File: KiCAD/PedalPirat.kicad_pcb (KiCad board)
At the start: 2 copper layers, 55 parts, among them IC1 IS31CS8979-QFLS2-TR, IC2 IS32IO1028A-GRLA2-TR

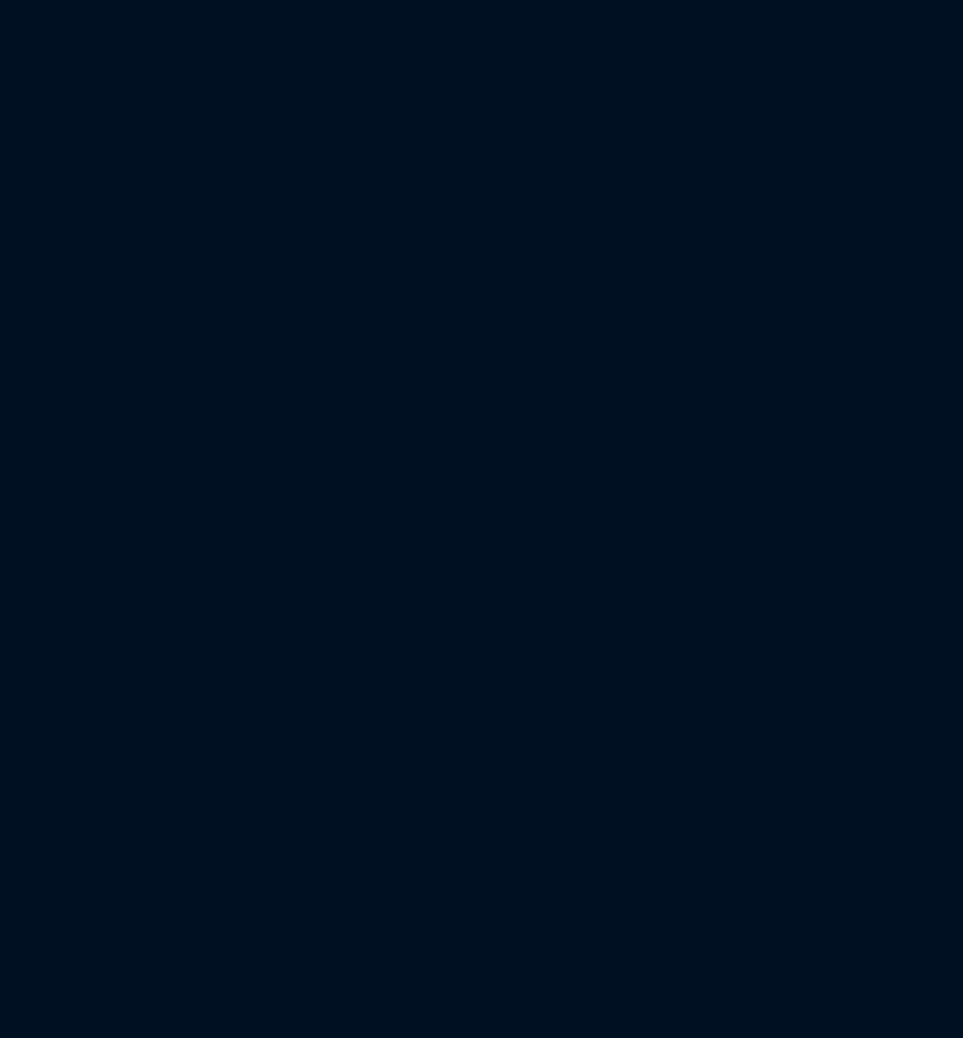
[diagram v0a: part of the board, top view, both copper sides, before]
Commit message: dasasd
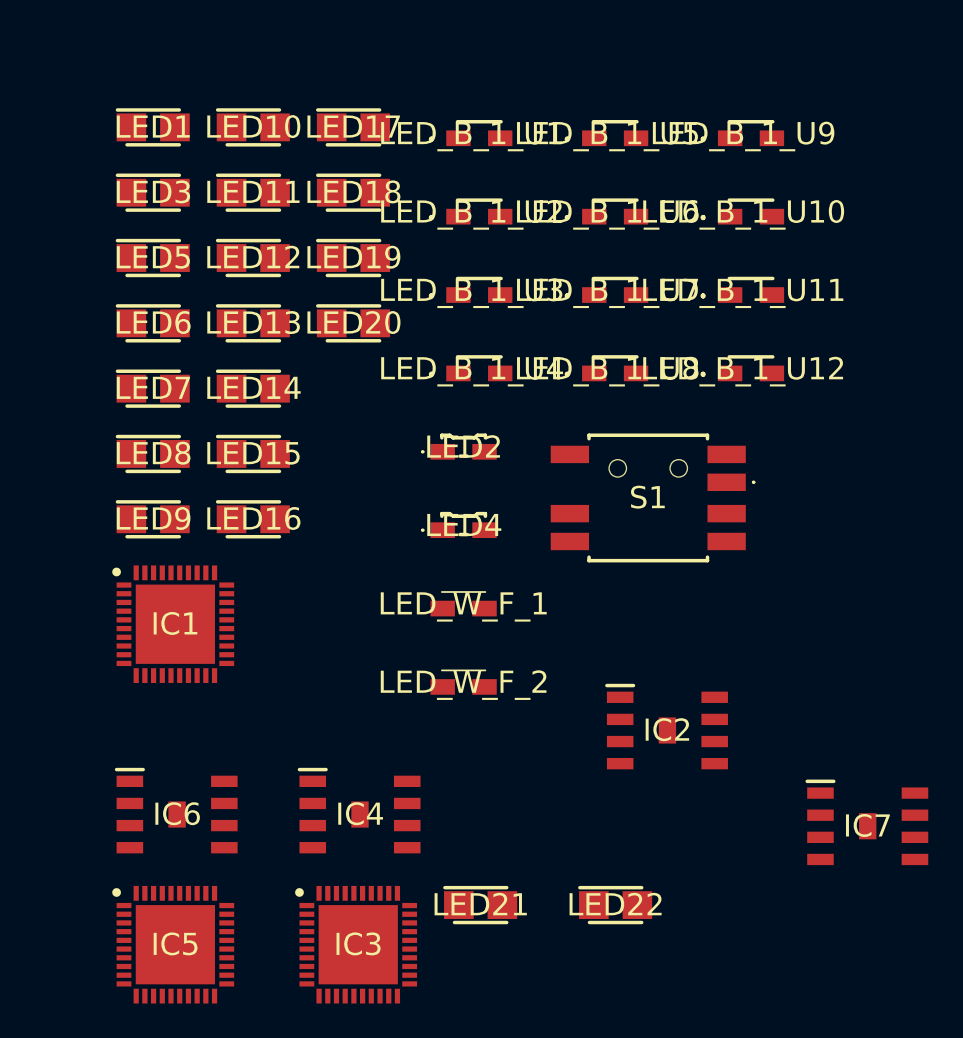
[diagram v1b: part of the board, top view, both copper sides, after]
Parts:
- added IC1: IS31CS8979-QFLS2-TR, SamacSys_Parts:QFN50P600X600X80-41N-D, F.Cu at (221.8, 97.4)
- added IC2: IS32IO1028A-GRLA2-TR, SamacSys_Parts:SOIC127P600X170-9N, F.Cu at (250.0, 103.5)
- added IC3: IS31CS8979-QFLS2-TR, SamacSys_Parts:QFN50P600X600X80-41N-D, F.Cu at (232.2, 115.8)
- added IC4: IS32IO1028A-GRLA2-TR, SamacSys_Parts:SOIC127P600X170-9N, F.Cu at (232.3, 108.3)
- added IC5: IS31CS8979-QFLS2-TR, SamacSys_Parts:QFN50P600X600X80-41N-D, F.Cu at (221.8, 115.8)
- added IC6: IS32IO1028A-GRLA2-TR, SamacSys_Parts:SOIC127P600X170-9N, F.Cu at (221.8, 108.3)
- added IC7: IS32LT3183A-GRLA3-TR, SamacSys_Parts:SOIC127P600X170-9N, F.Cu at (261.5, 109.0)
- added LED1: AA3021SESK_J3-TR, SamacSys_Parts:LEDM3020X150N, F.Cu at (220.5, 68.9)
- added LED10: AA3021SYSK_J3-TR, SamacSys_Parts:LEDM3020X150N, F.Cu at (226.2, 68.9)
- added LED11: AA3021SYSK_J3-TR, SamacSys_Parts:LEDM3020X150N, F.Cu at (226.2, 72.6)
- added LED12: AA3021SYSK_J3-TR, SamacSys_Parts:LEDM3020X150N, F.Cu at (226.2, 76.4)
- added LED13: AA3021SESK_J3-TR, SamacSys_Parts:LEDM3020X150N, F.Cu at (226.2, 80.1)
- added LED14: AA3021SYSK_J3-TR, SamacSys_Parts:LEDM3020X150N, F.Cu at (226.2, 83.9)
- added LED15: AA3021SYSK_J3-TR, SamacSys_Parts:LEDM3020X150N, F.Cu at (226.2, 87.6)
- added LED16: AA3021SYSK_J3-TR, SamacSys_Parts:LEDM3020X150N, F.Cu at (226.2, 91.4)
- added LED17: AA3021SYSK_J3-TR, SamacSys_Parts:LEDM3020X150N, F.Cu at (232.0, 68.9)
- added LED18: AA3021SYSK_J3-TR, SamacSys_Parts:LEDM3020X150N, F.Cu at (232.0, 72.6)
- added LED19: AA3021SYSK_J3-TR, SamacSys_Parts:LEDM3020X150N, F.Cu at (232.0, 76.4)
- added LED2: AA2810ASES_J3, SamacSys_Parts:AA2810ASESJ3, F.Cu at (238.3, 87.2)
- added LED20: AA3021SESK_J3-TR, SamacSys_Parts:LEDM3020X150N, F.Cu at (232.0, 80.1)
- added LED21: AA3021SYSK_J3-TR, SamacSys_Parts:LEDM3020X150N, F.Cu at (239.3, 113.5)
- added LED22: AA3021SYSK_J3-TR, SamacSys_Parts:LEDM3020X150N, F.Cu at (247.0, 113.5)
- added LED3: AA3021SESK_J3-TR, SamacSys_Parts:LEDM3020X150N, F.Cu at (220.5, 72.6)
- added LED4: AA2810ASES_J3, SamacSys_Parts:AA2810ASESJ3, F.Cu at (238.3, 91.8)
- added LED5: AA3021SESK_J3-TR, SamacSys_Parts:LEDM3020X150N, F.Cu at (220.5, 76.4)
- added LED6: AA3021SESK_J3-TR, SamacSys_Parts:LEDM3020X150N, F.Cu at (220.5, 80.1)
- added LED7: AA3021SYSK_J3-TR, SamacSys_Parts:LEDM3020X150N, F.Cu at (220.5, 83.9)
- added LED8: AA3021SYSK_J3-TR, SamacSys_Parts:LEDM3020X150N, F.Cu at (220.5, 87.6)
- added LED9: AA3021SYSK_J3-TR, SamacSys_Parts:LEDM3020X150N, F.Cu at (220.5, 91.4)
- added LED_B_1_U1: AA2810AQBS_D, SamacSys_Parts:AA2810AQBSD, F.Cu at (239.2, 69.5)
- added LED_B_1_U10: AA2810AQBS_D, SamacSys_Parts:AA2810AQBSD, F.Cu at (254.8, 74.0)
- added LED_B_1_U11: AA2810AQBS_D, SamacSys_Parts:AA2810AQBSD, F.Cu at (254.8, 78.5)
- added LED_B_1_U12: AA2810AQBS_D, SamacSys_Parts:AA2810AQBSD, F.Cu at (254.8, 83.0)
- added LED_B_1_U2: AA2810AQBS_D, SamacSys_Parts:AA2810AQBSD, F.Cu at (239.2, 74.0)
- added LED_B_1_U3: AA2810AQBS_D, SamacSys_Parts:AA2810AQBSD, F.Cu at (239.2, 78.5)
- added LED_B_1_U4: AA2810AQBS_D, SamacSys_Parts:AA2810AQBSD, F.Cu at (239.2, 83.0)
- added LED_B_1_U5: AA2810AQBS_D, SamacSys_Parts:AA2810AQBSD, F.Cu at (247.0, 69.5)
- added LED_B_1_U6: AA2810AQBS_D, SamacSys_Parts:AA2810AQBSD, F.Cu at (247.0, 74.0)
- added LED_B_1_U7: AA2810AQBS_D, SamacSys_Parts:AA2810AQBSD, F.Cu at (247.0, 78.5)
- added LED_B_1_U8: AA2810AQBS_D, SamacSys_Parts:AA2810AQBSD, F.Cu at (247.0, 83.0)
- added LED_B_1_U9: AA2810AQBS_D, SamacSys_Parts:AA2810AQBSD, F.Cu at (254.8, 69.5)
- added LED_W_F_1: AA2810AVW1S, SamacSys_Parts:AA2810AVW1S, F.Cu at (238.3, 96.2)
- added LED_W_F_2: AA2810AVW1S, SamacSys_Parts:AA2810AVW1S, F.Cu at (238.3, 100.7)
- added S1: 228EMVARGBFR, SamacSys_Parts:228EMVARGBFR, F.Cu at (248.9, 90.2)
